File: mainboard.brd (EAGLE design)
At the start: 93.9 x 67.6 mm, 46 parts, among them IC1 DS1307, IC2 LM2596S, J1 AVR_SPI_PRG_6PTH, Q1 32.768 kHz, U1 ATMEGA328P, U2 3.3V, U3 5V, U4 MMA7660FCR1

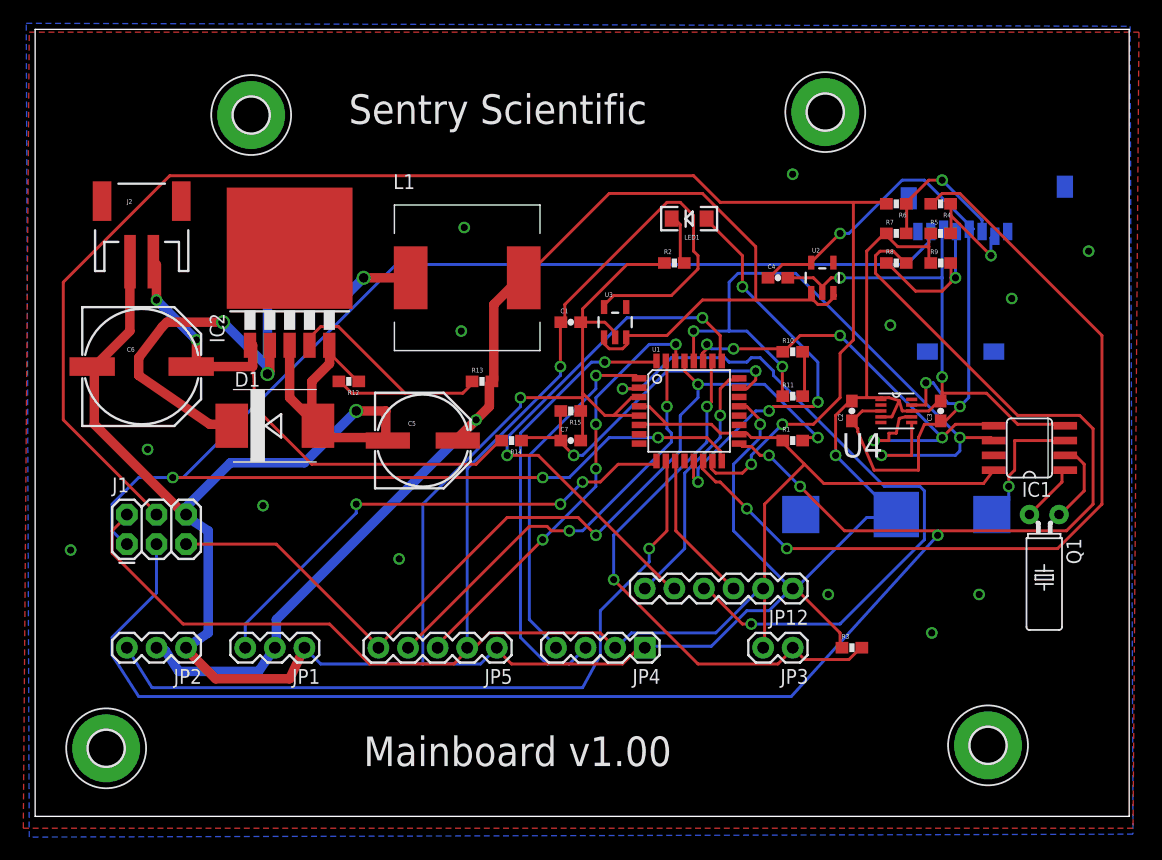
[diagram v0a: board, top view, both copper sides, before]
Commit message: Updates
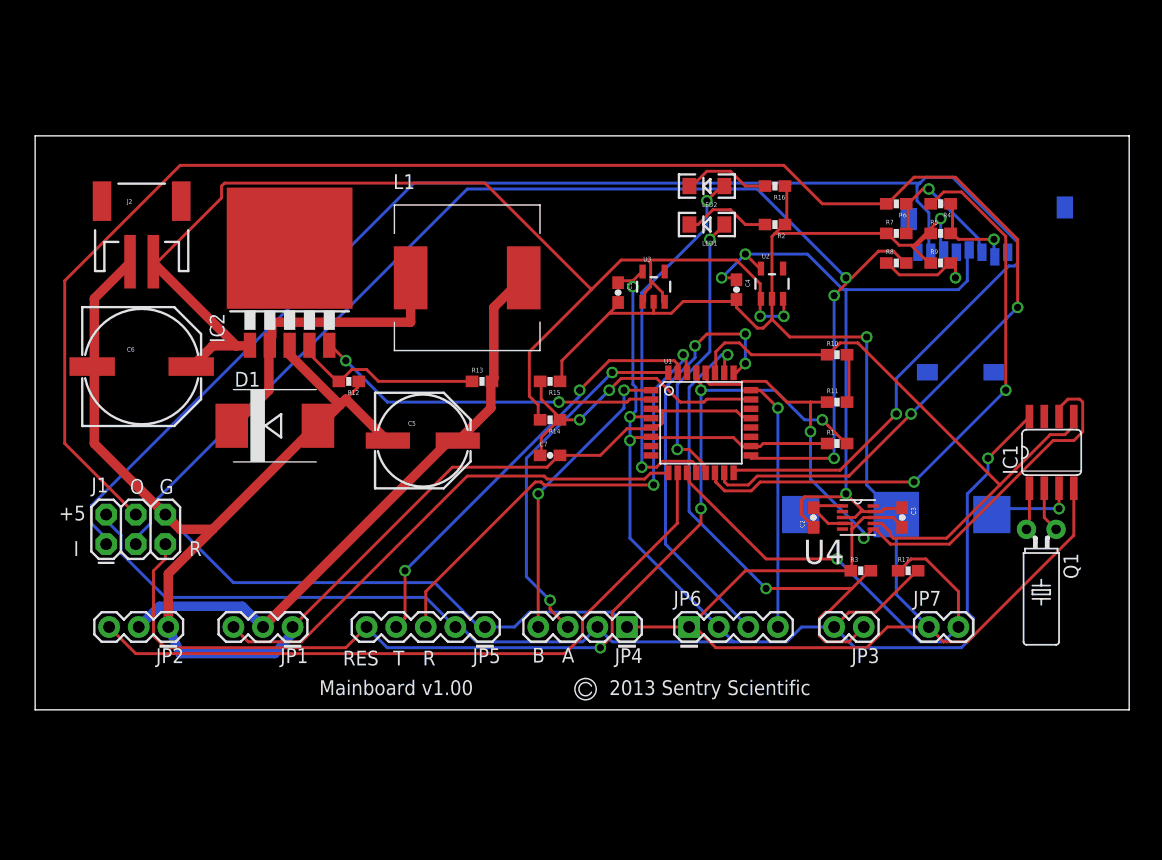
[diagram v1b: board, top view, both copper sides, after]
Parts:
- removed H1, H2, H3, H4: MOUNT-PAD-ROUND3.0, holes:3,0-PAD
- removed JP12: Extra, SparkFun-Connectors:1X06
- added JP6: Extra, SparkFun-Connectors:1X04
- added JP7: MAIN_SW, SparkFun-Connectors:1X02
- added LED2: (no value), SparkFun-LED:LED-1206
- added R16: 100, SparkFun-Resistors:0603-RES
- added R17: 10k, SparkFun-Resistors:0603-RES
- moved C2 9.72 mm to (68.6, 27.4)
- moved C3 9.72 mm to (76.2, 27.4), turned to 270 degrees
- moved U4 9.72 mm to (72.4, 27.4)
- moved R2 9.25 mm to (65.3, 52.6), turned to 180 degrees
- moved R3 6.65 mm to (72.6, 22.9)
- moved JP3 6.35 mm to (72.9, 18.0)
- moved C1 4.79 mm to (51.8, 46.7), turned to 270 degrees
- moved U3 4.49 mm to (54.9, 47.2)
- moved U2 4.35 mm to (65.0, 47.5)
- moved R11 3.84 mm to (70.6, 37.3)
- moved R1 3.82 mm to (70.6, 33.8)
- moved R10 3.82 mm to (70.6, 41.4)
- moved R14 3.75 mm to (46.0, 35.8)
- moved C4 3.70 mm to (62.0, 47.0), turned to 270 degrees
- moved R15 3.10 mm to (46.0, 39.1)
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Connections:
- removed net D4: JP12.4, U1.2
- removed net D7: JP12.3, U1.11
- new net 6V_ON: IC2.5, U1.2
- new net MAIN_SW: JP7.2, R17.1, U1.11
- new net N$12: LED2.C, R16.2
- new net N$13: LED2.A, U1.12
- net +5V: now also JP6.2, R17.2; no longer JP12.2
- net +6V: no longer U2.1, U2.3, U3.1, U3.3
- net A1: now also JP6.4; no longer JP12.6
- net A2: now also JP6.3; no longer JP12.5
- net BAT+: now also U2.1, U2.3, U3.1, U3.3
- net GND: now also JP6.1, JP7.1, R16.1; no longer IC2.5, JP12.1
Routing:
- net D4: track 61.1 -> 0.00 mm, vias 2 -> 0
- net BAT+: track 45.5 -> 103.9 mm
- net +6V: track 109.2 -> 51.9 mm, vias 1 -> 0
- net SCK: track 160.2 -> 107.8 mm
- net MAIN_SW: track 0.00 -> 40.1 mm, vias 0 -> 1
- net N$13: track 0.00 -> 32.8 mm, vias 0 -> 2
- net 6V_ON: track 0.00 -> 29.7 mm, vias 0 -> 2
- net SD_CS: track 73.9 -> 51.3 mm
- net N$10: track 47.6 -> 26.1 mm, vias 3 -> 0
- net MOSI: track 130.9 -> 151.2 mm
- net GND: track 338.8 -> 354.2 mm, vias 19 -> 2
- net +5V: track 183.9 -> 170.3 mm, vias 1 -> 4
- net RESET: track 76.8 -> 90.3 mm, vias 3 -> 4
- net D7: track 13.0 -> 0.00 mm
- net SDA: track 42.1 -> 55.1 mm, vias 5 -> 0
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- removed copper zone on layer 1, net GND
- removed copper zone on layer 16, net GND
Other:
- board size 93.9 x 67.6 mm -> 93.9 x 49.3 mm
- board text added: "+5"
- board text added: "2013 Sentry Scientific"
- board text added: "A"
- board text added: "B"
- board text added: "G"
- board text added: "I"
- board text added: "O"
- board text added: "R"
- board text added: "RES"
- board text added: "T"
- board text removed: "Sentry Scientific"
